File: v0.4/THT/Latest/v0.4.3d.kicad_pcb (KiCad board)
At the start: 2 copper layers, 100 x 100 mm, 134 parts, among them IC3 Trig Cond Socket, J1 Conn_01x05, J2 Conn_01x06, J3 Conn_01x02, J4 Conn_02x20_Counter_Clockwise, J5 Conn_01x04, J6 Conn_01x05, J8 Conn_01x03, Q1 Q_NMOS_GDS, Q2 Q_NMOS_GDS, Q3 Q_NMOS_GDS, Q4 Q_NMOS_GDS, Q5 Q_NMOS_GDSD, Q6 Q_NMOS_GDSD, U1 SP721, U2 TC4424A, U3 SP721, U4 TC4424A, U5 MPX4250, U6 ULN2003, U8 LM2940S-5.0

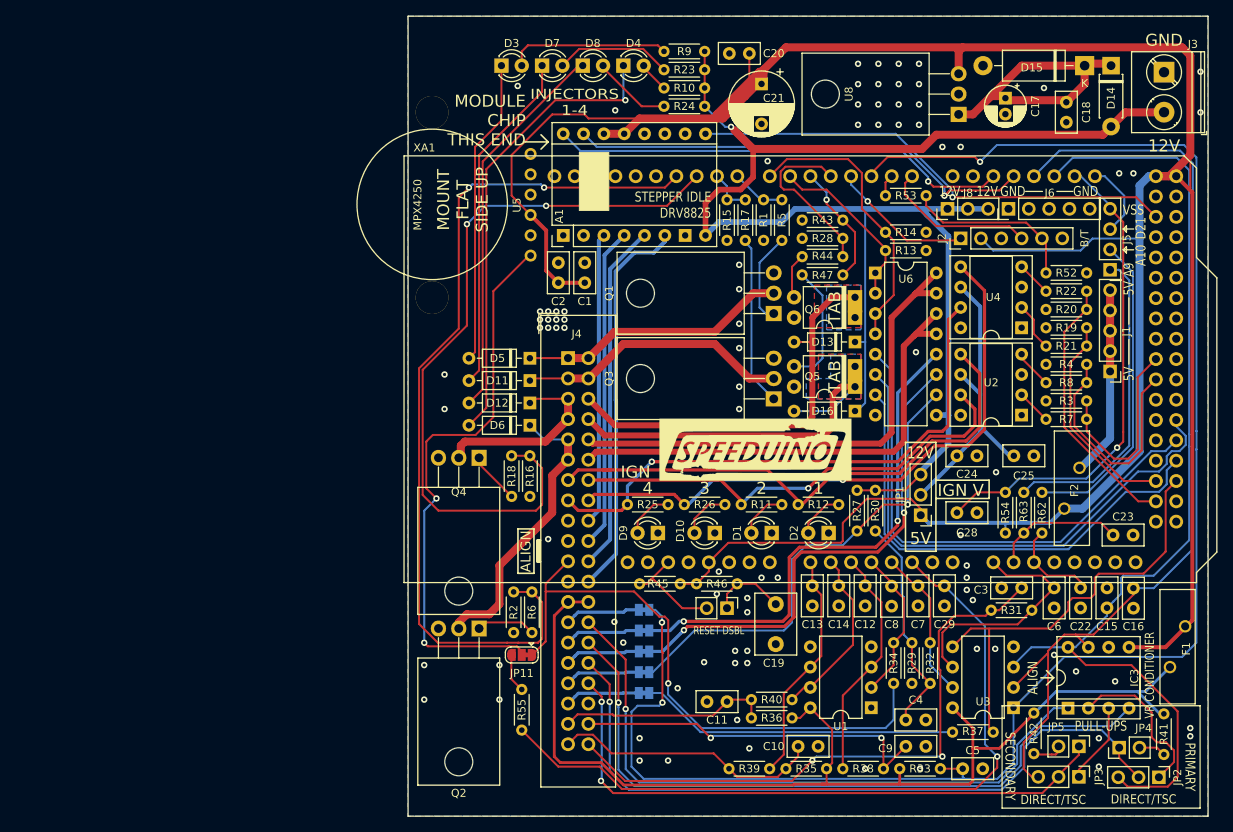
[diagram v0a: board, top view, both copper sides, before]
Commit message: kicad work
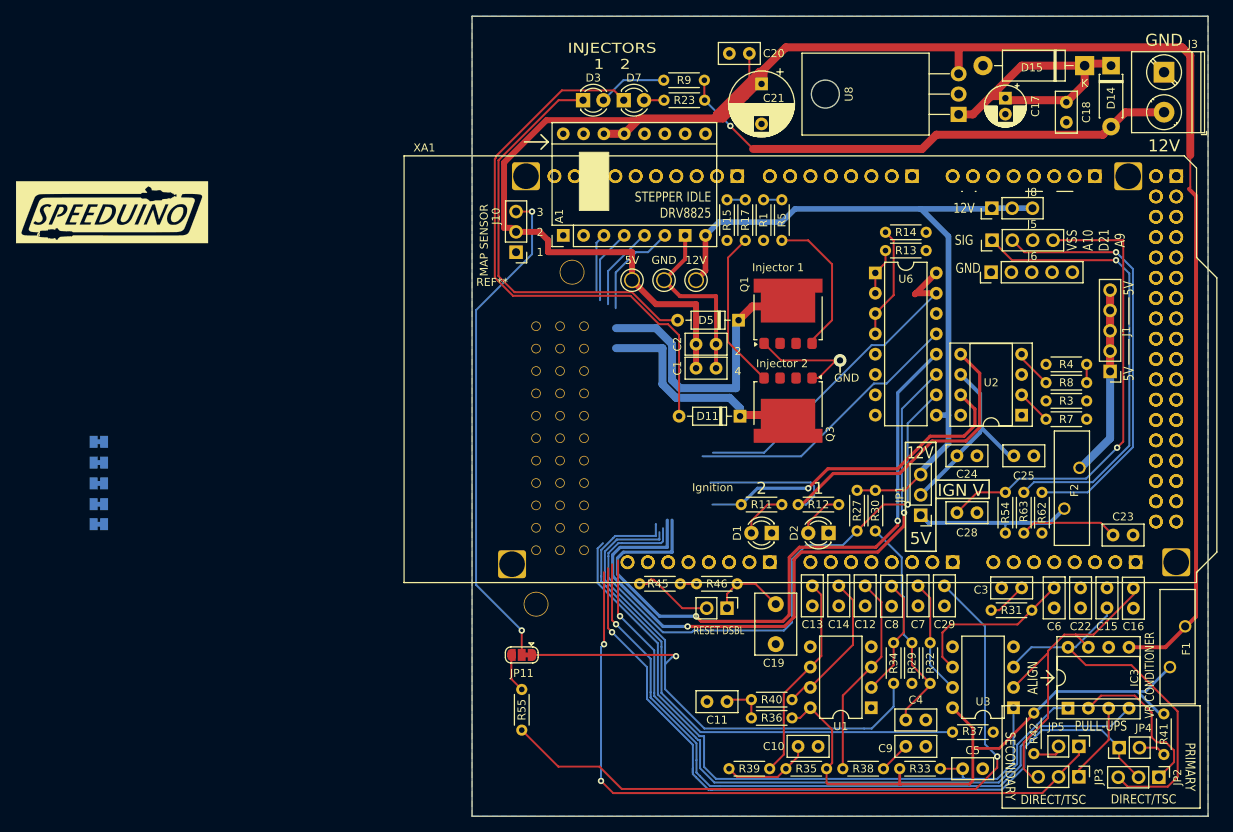
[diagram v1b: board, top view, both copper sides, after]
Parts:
- removed D10, D4, D8, D9: LED, LED_THT:LED_D3.0mm
- removed D12, D13, D16, D6: D, Diode_THT:D_DO-35_SOD27_P7.62mm_Horizontal
- removed J2: Conn_01x06, Connector_PinHeader_2.54mm:PinHeader_1x06_P2.54mm_Vertical
- removed J4: Conn_02x20_Counter_Clockwise, Connector_IDC:IDC-Header_2x20_P2.54mm_Vertical
- removed Q2, Q4: Q_NMOS_GDS, Package_TO_SOT_THT:TO-220-3_Horizontal_TabDown
- removed Q5, Q6: Q_NMOS_GDSD, Package_DIP:Vishay_HVM-DIP-3_W7.62mm
- removed R10, R24, R25, R26: 2.4k, Resistor_THT:R_Axial_DIN0204_L3.6mm_D1.6mm_P5.08mm_Horizontal
- removed R16, R19, R2, R20, R28, R43: 100k, Resistor_THT:R_Axial_DIN0204_L3.6mm_D1.6mm_P5.08mm_Horizontal
- removed R18, R21, R22, R44, R47, R53, R6: 1k, Resistor_THT:R_Axial_DIN0204_L3.6mm_D1.6mm_P5.08mm_Horizontal
- removed R52: 2k, Resistor_THT:R_Axial_DIN0204_L3.6mm_D1.6mm_P5.08mm_Horizontal
- removed U4: TC4424A, Package_DIP:DIP-8_W7.62mm_Socket
- removed U5: MPX4250, Misc:MPX4250
- added 12V: TestPoint_Keystone_5000-5004_Miniature, TestPoint:TestPoint_Keystone_5000-5004_Miniature, F.Cu at (146.5, 70.0)
- added 5V: TestPoint_Keystone_5000-5004_Miniature, TestPoint:TestPoint_Keystone_5000-5004_Miniature, F.Cu at (138.5, 70.0)
- added ?: , , F.Cu at (123.5, 105.5)
- added ?: , , F.Cu at (125.0, 57.0)
- added ?: , , F.Cu at (206.5, 105.5)
- added ?: , , F.Cu at (200.0, 57.0)
- added GND: TestPoint_Keystone_5000-5004_Miniature, TestPoint:TestPoint_Keystone_5000-5004_Miniature, F.Cu at (142.5, 70.0)
- added J10: Conn_01x03, Connector_PinHeader_2.54mm:PinHeader_1x03_P2.54mm_Vertical, F.Cu at (124.0, 66.5)
- added REF**: 6189-7106, user-made:6189-7106, F.Cu at (126.5, 75.8)
- added REF**: PinHeader_1x08_P2.54mm_Vertical, Connector_PinHeader_2.54mm:PinHeader_1x08_P2.54mm_Vertical, B.Cu at (201.4, 105.2)
- added REF**: PinHeader_1x08_P2.54mm_Vertical, Connector_PinHeader_2.54mm:PinHeader_1x08_P2.54mm_Vertical, B.Cu at (173.5, 57.0)
- added REF**: PinHeader_1x08_P2.54mm_Vertical, Connector_PinHeader_2.54mm:PinHeader_1x08_P2.54mm_Vertical, B.Cu at (155.7, 105.2)
- added REF**: PinHeader_1x08_P2.54mm_Vertical, Connector_PinHeader_2.54mm:PinHeader_1x08_P2.54mm_Vertical, B.Cu at (178.6, 105.2)
- added REF**: PinHeader_1x08_P2.54mm_Vertical, Connector_PinHeader_2.54mm:PinHeader_1x08_P2.54mm_Vertical, B.Cu at (196.3, 57.0)
- added REF**: PinHeader_1x10_P2.54mm_Vertical, Connector_PinHeader_2.54mm:PinHeader_1x10_P2.54mm_Vertical, B.Cu at (151.7, 57.0)
- added REF**: PinHeader_2x18_P2.54mm_Vertical, Connector_PinHeader_2.54mm:PinHeader_2x18_P2.54mm_Vertical, B.Cu at (206.5, 57.0)
- Q1, Q3: value Q_NMOS_GDS -> LFPAK88; footprint Package_TO_SOT_THT:TO-220-3_Horizontal_TabDown -> Package_TO_SOT_SMD:LFPAK88
- moved G*** 85.7 mm to (73.5, 61.5)
- moved JP10 72.1 mm to (71.8, 98.0)
- moved JP7 72.1 mm to (71.8, 90.2)
- moved JP8 72.1 mm to (71.8, 92.8)
- moved JP9 72.1 mm to (71.8, 95.4)
- moved JP6 69.0 mm to (71.8, 100.5)
- moved D11 26.6 mm to (152.0, 87.0)
- moved D5 26.5 mm to (151.8, 75.0)
- moved C2 22.2 mm to (149.0, 78.0), turned to 180 degrees
- moved C1 21.1 mm to (149.0, 81.0), turned to 180 degrees
- moved J5 15.2 mm to (183.5, 65.0), turned to 90 degrees
- moved D7 11.1 mm to (137.5, 47.5)
- moved D3 11.1 mm to (132.4, 47.5)
- moved J6 8.21 mm to (183.4, 69.0)
- moved J8 5.54 mm to (183.5, 61.0)
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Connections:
- Q1 pad 1: Net-(Q1-Pad1) -> GND
- Q1 pad 2: INJ-1-OUT -> (no net)
- Q1 pad 3: GND -> (no net)
- Q3 pad 1: Net-(Q3-Pad1) -> GND
- Q3 pad 2: INJ-2-OUT -> (no net)
- Q3 pad 3: GND -> (no net)
- XA1 pad D0: MCU-D0 -> (no net)
- XA1 pad D1: MCU-D1 -> (no net)
- XA1 pad D3: MCU-D3 -> (no net)
- XA1 pad D4: MCU-D4 -> (no net)
- XA1 pad D5: MCU-D5 -> (no net)
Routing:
- net ADC-Clamp-7: track 215.0 -> 85.3 mm, vias 3 -> 0
- net MCU-D11: track 109.2 -> 0.00 mm, vias 2 -> 0
- net MCU-D10: track 92.4 -> 0.00 mm, vias 2 -> 0
- net VDD: track 355.9 -> 266.0 mm
- net ADC-Clamp-9: track 128.8 -> 49.1 mm
- net ADC-Clamp-8: track 120.5 -> 40.9 mm
- net IGN-3-OUT: track 75.8 -> 0.00 mm, vias 1 -> 0
- net O2_Sensor: track 75.9 -> 4.97 mm, vias 2 -> 0
- net IGN-4-OUT: track 69.2 -> 0.00 mm, vias 1 -> 0
- net MCU-D45: track 67.7 -> 0.00 mm
- net MCU-D47: track 64.4 -> 0.00 mm
- net MCU-D24: track 61.1 -> 0.00 mm, vias 1 -> 0
- net MCU-D49: track 60.7 -> 0.00 mm
- net VDDA: track 136.4 -> 77.6 mm
- net MCU-D17: track 58.6 -> 0.00 mm, vias 1 -> 0
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- removed copper zone on F.Cu, net GND
- removed copper zone on B.Cu, net HC-2-OUT
- removed copper zone on F.Cu, net HC-2-OUT
- removed copper zone on B.Cu, net IDLE-OUT
- removed copper zone on F.Cu, net IDLE-OUT
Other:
- board size 100 x 100 mm -> 92 x 100 mm
- net class Default removed
- board text added: "1"
- board text added: "2"
- board text added: "3"
- board text added: "4"
- board text added: "INJECTORS 1 2"
- board text added: "Ignition"
- board text added: "Injector 1"
- board text added: "Injector 2"
- board text added: "MAP SENSOR"
- board text added: "REV 0.0.1 - diarmuid kelly 2025"
- board text added: "SIG"
- board text removed: "B/T"
- board text removed: "IGN"
- board text removed: "INJECTORS 1-4"
- board text removed: "MODULE CHIP THIS END"
- board text removed: "MOUNT FLAT SIDE UP"
- board text removed: "TAB"
